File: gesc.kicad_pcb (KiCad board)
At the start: 4 copper layers, 111 x 111 mm, 161 parts, among them J1 Conn_01x06, J10 PHASE_C, J11 PHASE_B, J13 T-Motor, J14 Conn_01x03, J15 EXT_OFF, J2 Conn_01x06, J3 Conn_01x06, J4 Conn_01x05, J5 Conn_01x03, J6 USB_B_Mini, J7 BAT+, J8 BAT-, J9 PHASE_A, Q1 BSC070N10NS5, Q2 BSC070N10NS5, Q3 BSC070N10NS5, Q4 BSC070N10NS5, Q5 BSC070N10NS5, Q6 BSC070N10NS5, U1 STM32F405RGTx, U10 LM5008MM, U11 SN74LVC1G66DBVR, U12 2ED2304S06F, U13 SN74LVC1G66DBVR, U14 AQY282S, U15 2ED2304S06F, U16 EYSGJNZWY, U17 LMR12010YMKE_NOPB, U2 SN74LVC1G66DBVR, U3 2ED2304S06F, U4 INA240A1, U5 INA240A1, U6 INA240A1, U7 SN74LVC1G66DBVR, U8 SN74LVC1G66DBVR, U9 SN74LVC1G66DBVR, Y1 X50328MSB2GI

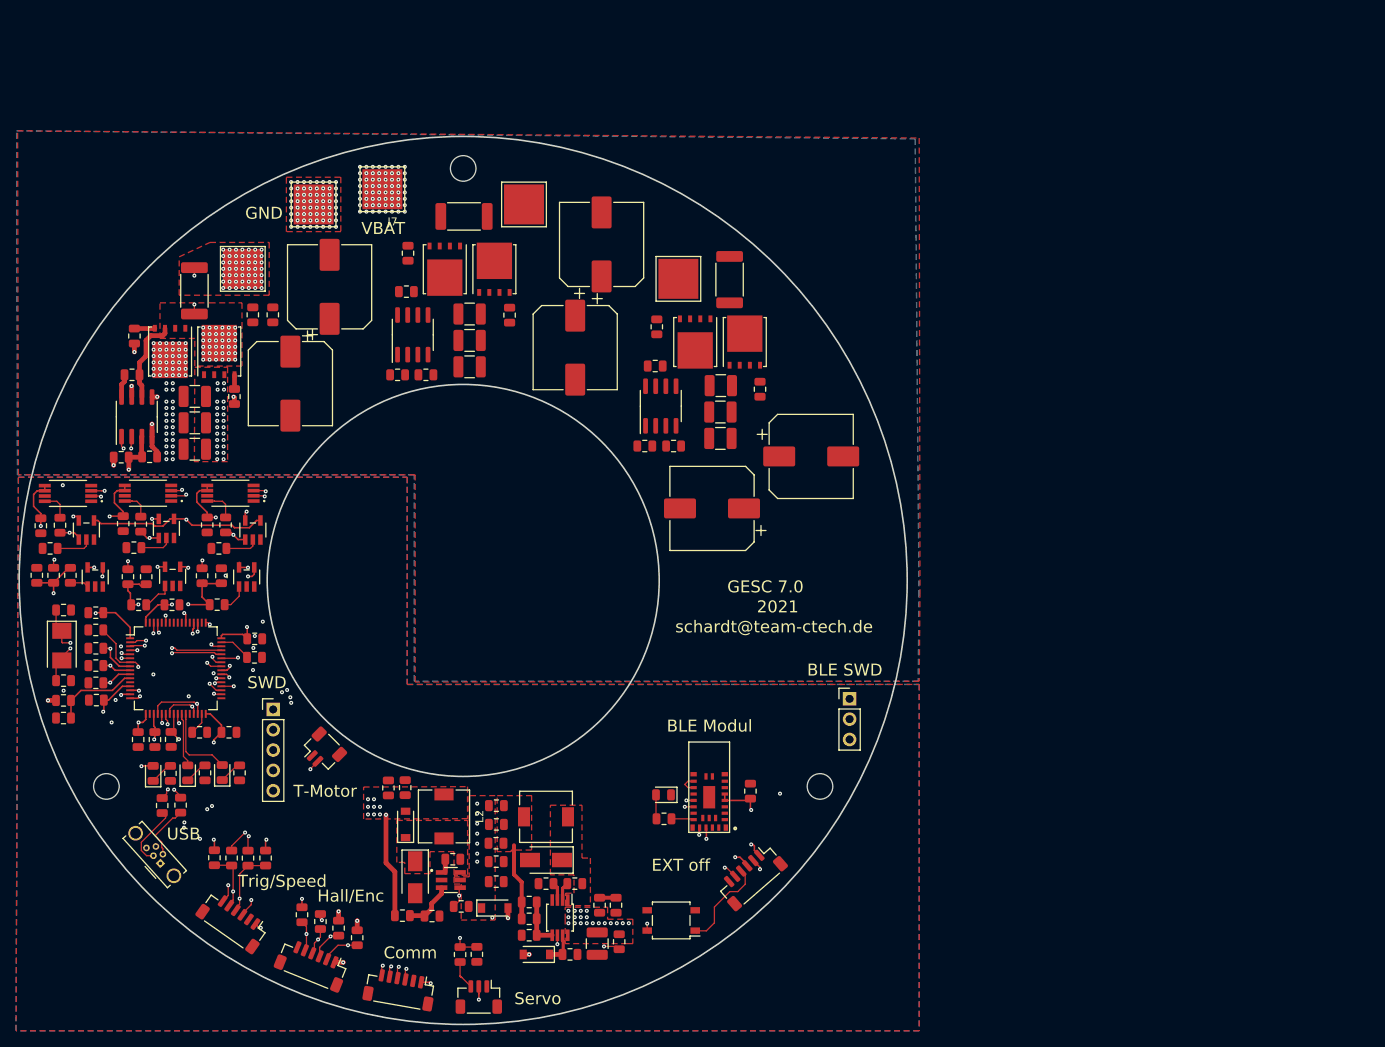
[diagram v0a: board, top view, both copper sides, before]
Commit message: save
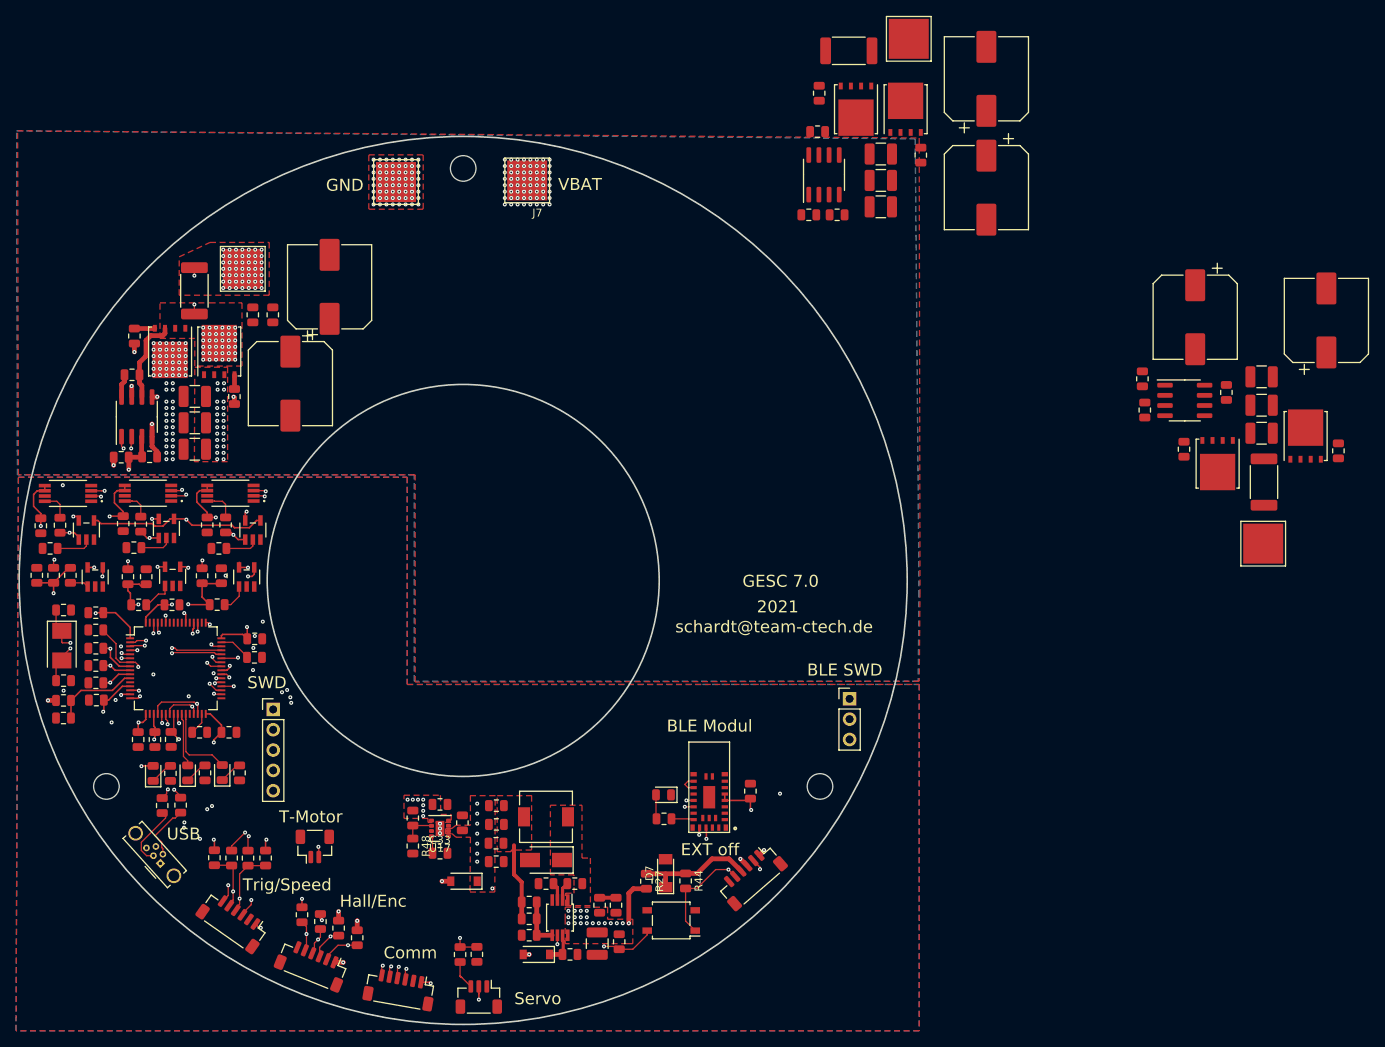
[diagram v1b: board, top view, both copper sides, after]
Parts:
- removed C50: 22u0/25V, Capacitor_SMD:C_0805_2012Metric
- removed D8: SS210, Diode_SMD:D_SMA
- removed L2: 15u0, Inductor_SMD:L_6.3x6.3_H3
- added R48: 110k, Resistor_SMD:R_0805_2012Metric, F.Cu at (93.7, 133.2)
- C33: value 100n -> 3n30
- D7: value B5819W -> ZPD12; footprint Diode_SMD:D_SOD-123 -> Diode_SMD:D_MiniMELF
- R15: value 100k -> 110k
- R27: value 11k0 -> 3k30
- R34: value 11k0 -> 330k
- R44: value 33k0 -> 2k10
- U17: value LMR12010YMKE_NOPB -> TPS82140; footprint gesc:SOT95P280X110-6N -> Package_LGA:Texas_SIL0008D_MicroSiP-8-1EP_2.8x3mm_P0.65mm_EP1.1x1.9mm
- moved R25 86.6 mm to (209.4, 83.8), turned to 90 degrees
- moved J10 80.2 mm to (200.0, 95.4)
- moved Q3 77.2 mm to (205.3, 81.9), turned to 90 degrees
- moved C32 71.5 mm to (195.4, 76.5), turned to 270 degrees
- moved R31 71.4 mm to (200.1, 87.7)
- moved C52 68.1 mm to (199.8, 74.5), turned to 180 degrees
- moved C43 67.9 mm to (199.8, 81.6), turned to 180 degrees
- moved C36 67.7 mm to (199.8, 78.1), turned to 180 degrees
- moved C61 66.6 mm to (207.9, 67.5), turned to 90 degrees
- moved U15 65.5 mm to (190.2, 77.5), turned to 0 degrees
- moved C62 65.0 mm to (191.5, 67.1), turned to 270 degrees
- moved C58 62.8 mm to (184.9, 74.8), turned to 90 degrees
- moved Q4 61.0 mm to (194.3, 85.4), turned to 270 degrees
- moved C29 59.1 mm to (185.2, 78.7), turned to 270 degrees
- moved C22 55.2 mm to (146.7, 54.3)
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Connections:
- C33 pad 2: Net-(C33-Pad2) -> GND
- D7 pad 1: Net-(C33-Pad2) -> /Driver/V_AUX
- D7 pad 2: VCC -> GND
- J15 pad 4: /Driver/EN_3V3 -> /Driver/V_AUX
- R12 pad 1: /Driver/EN_12V -> Net-(R12-Pad1)
- R27 pad 1: +12V -> /Driver/V_AUX
- R27 pad 2: Net-(R27-Pad2) -> VBAT
- R34 pad 1: GND -> VCC
- R44 pad 1: VCC -> /Driver/V_AUX
- R44 pad 2: Net-(R34-Pad2) -> /Driver/EN_12V
- U10 pad 6: /Driver/EN_12V -> Net-(R12-Pad1)
- U14 pad 1: /Driver/EN_3V3 -> /Driver/EN_12V
- U14 pad 4: Net-(R27-Pad2) -> Net-(R12-Pad1)
- U17 pad 1: Net-(C33-Pad1) -> (no net)
- U17 pad 2: GND -> +12V
- U17 pad 3: Net-(R34-Pad2) -> GND
- U17 pad 4: Net-(R27-Pad2) -> VCC
- U17 pad 5: +12V -> VCC
- U17 pad 6: Net-(C33-Pad2) -> Net-(R34-Pad2)
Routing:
- net Net-(R27-Pad2): track 28.9 -> 0.00 mm, vias 2 -> 0
- net /Driver/EN_12V: track 30.0 -> 13.7 mm, vias 3 -> 1
- net /Driver/V_AUX: track 0.00 -> 15.0 mm
- net Net-(R12-Pad1): track 0.00 -> 14.1 mm, vias 0 -> 2
- net VCC: track 94.2 -> 80.4 mm, vias 38 -> 36
- net VBUS: track 50.0 -> 37.2 mm
- net /Driver/EN_3V3: track 10.9 -> 0.00 mm
- net +12V: track 137.0 -> 141.6 mm
- net VBAT: track 88.2 -> 92.0 mm
- net Net-(R34-Pad2): track 6.28 -> 3.98 mm
- net /MCU/TEMP_MOTOR: track 52.6 -> 50.3 mm
- net /MCU/SERVO: track 66.7 -> 68.7 mm
- net GND: vias 90 -> 93
- removed copper zone on F.Cu, net Net-(C33-Pad2)
